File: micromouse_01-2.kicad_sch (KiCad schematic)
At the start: 64 parts, among them IC6 PCA9632TK,118, J1 Conn_01x02_Pin, M3 Fan_Motor, Q1 MCM3400A-TP, Q2 MCM3400A-TP, Q3 MCM3400A-TP, Q4 Q_PMOS_GSD, Q5 Q_PMOS_GSD, Q6 Q_PMOS_GSD, SW3 SSSS810701, U1 SMT-0440-S-R, U2 LBR-127HLD, U3 LBR-127HLD, U4 LBR-127HLD, U5 LBR-127HLD, U6 LXDC55FAAA-203, U7 MCP73831-2-OT, U8 WS2812-2020

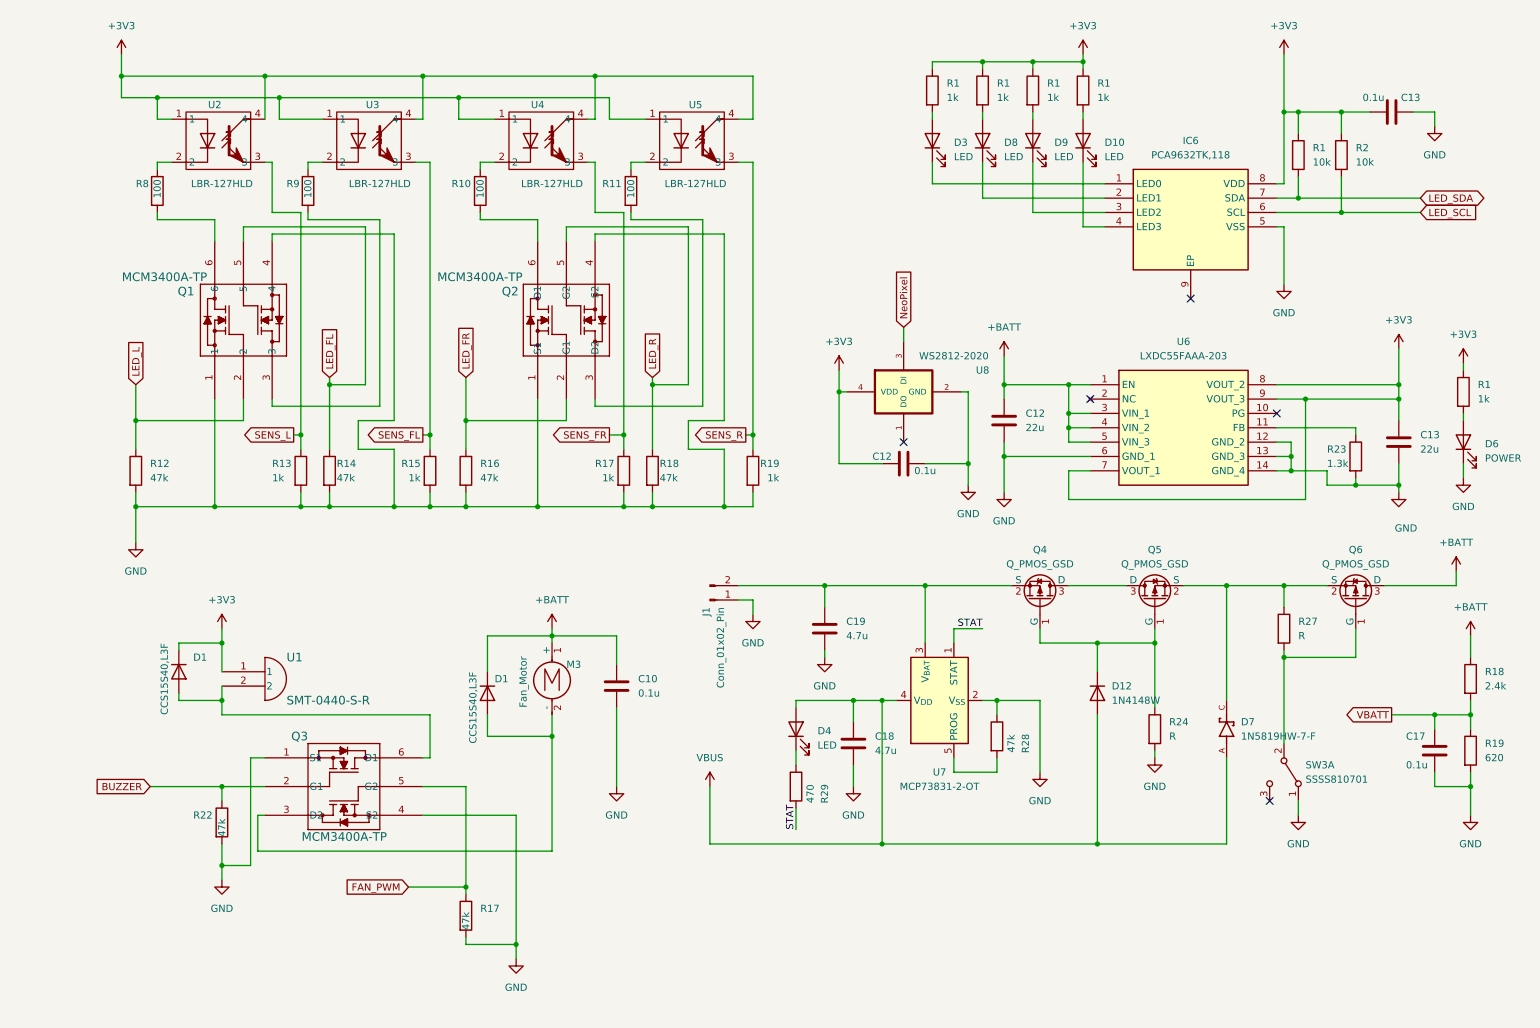
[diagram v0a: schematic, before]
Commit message: [update]けっこう線引いた
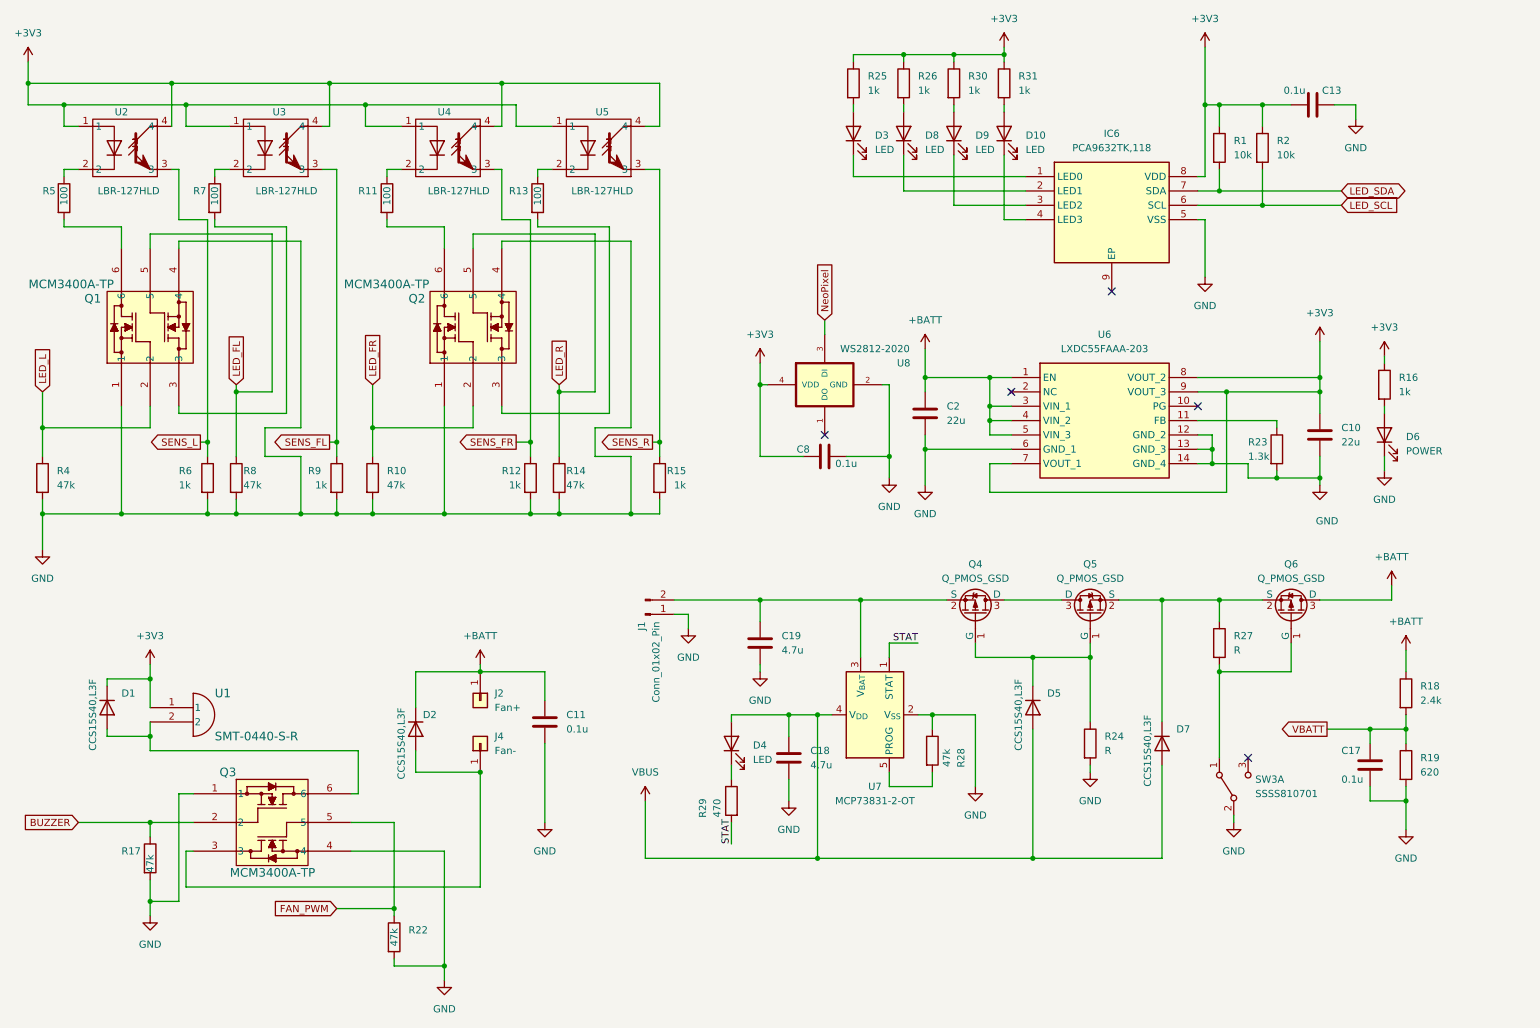
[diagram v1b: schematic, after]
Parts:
- removed D12: 1N4148W, Diode_SMD:D_SOD-123, symbol Diode:1N4148W
- removed D7: 1N5819HW-7-F, footprints:SOD3715X145N, symbol 1N5819HW-7-F:1N5819HW-7-F
- removed M3: Fan_Motor, footprints:MK06-4.5, symbol Motor:Motor_DC
- added D5, D7: CCS15S40,L3F, footprints:SOD-963 CST2C_TOS, symbol Diode:1N4148W
- added J2: Fan+, footprints:Pad_1, symbol Connector_Generic:Conn_01x01
- added J4: Fan-, footprints:Pad_1, symbol Connector_Generic:Conn_01x01
- J1: footprint footprints:power_SMD -> footprints:MK06-4.5
- Q1, Q2, Q3: footprint footprints:DFN2020-6L_MCE -> DFN2020-6L_MCE
- renumbered C13 to C10, C10 to C11, C12 to C2, C12 to C8, D1 to D2, R16 to R10, R10 to R11, R17 to R12, R11 to R13, R18 to R14, R19 to R15, R1 to R16, R22 to R17, R17 to R22, R1 to R25, R1 to R26, R1 to R30, R1 to R31, R12 to R4, R8 to R5, R13 to R6, R9 to R7, R14 to R8, R15 to R9
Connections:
- net +BATT: now also J2.1 (Pin_1)
- net GND: now also SW3.2 (B); no longer SW3.1 (A)
- net VBUS: now also D5.2 (A), D7.2 (A)
- net at D2.2 (A), Q3.3: now also J4.1 (Pin_1)
- net at Q6.1 (G), R27.2: now also SW3.1 (A); no longer SW3.2 (B)
- net at Q5.2 (S), Q6.2 (S), R27.1: now also D7.1 (K)
- net at Q4.1 (G), Q5.1 (G), R24.1: now also D5.1 (K)
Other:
- moved on the sheet: C10, C11, C13, C17, C18, C19, C2, C8, D1, D10, D2, D3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
